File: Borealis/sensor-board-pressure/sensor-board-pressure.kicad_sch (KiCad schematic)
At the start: 3 parts, among them J1 Conn_01x06_Pin, J2 Conn_01x08_Pin (BMP390)

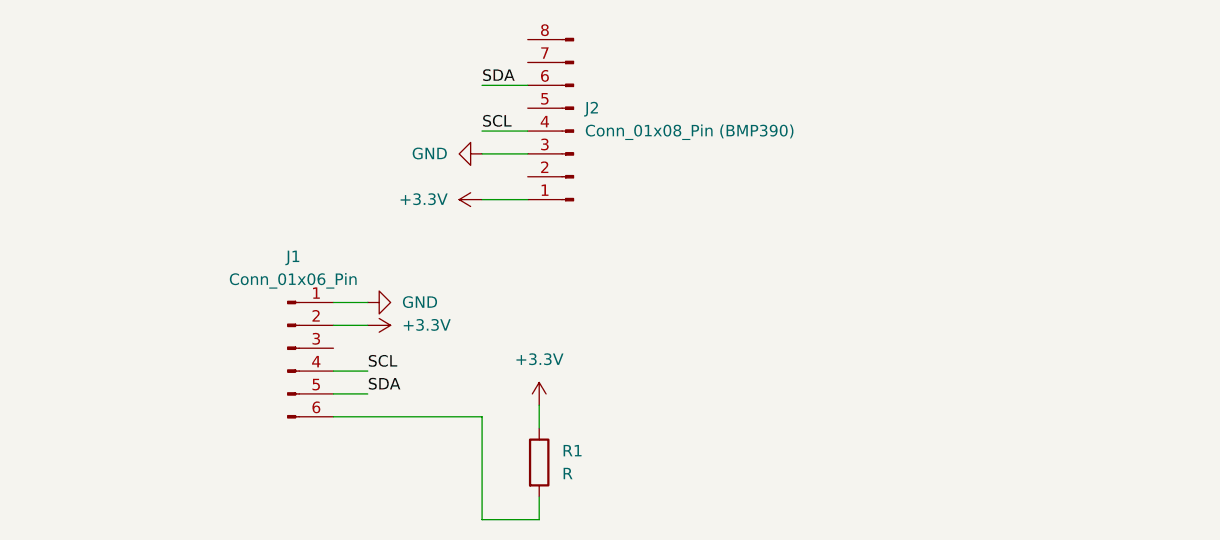
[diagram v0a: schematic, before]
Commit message: Updating changes
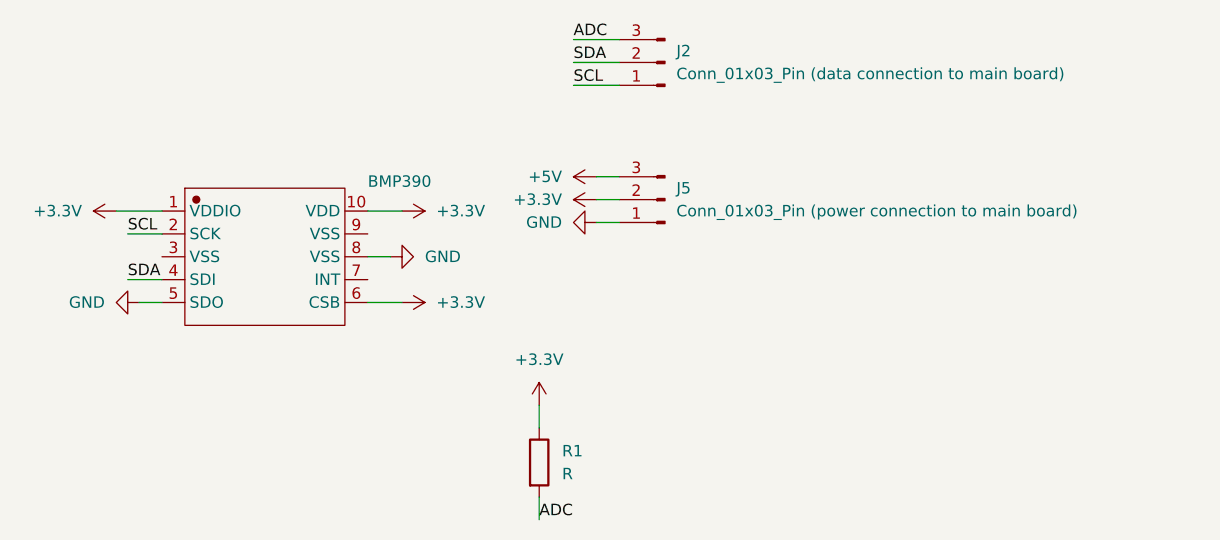
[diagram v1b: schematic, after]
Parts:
- removed J1: Conn_01x06_Pin, Connector_PinHeader_2.54mm:PinHeader_1x06_P2.54mm_Vertical, symbol Connector:Conn_01x06_Pin
- removed J2: Conn_01x08_Pin (BMP390), Adafruit BMP390:1X08_ROUND_70, symbol Connector:Conn_01x08_Pin
- added BMP390: ~, Adafruit BMP390:BMP388, symbol BMP390_2025-12-25-altium-import:root_0_BMP390_
- added J2: Conn_01x03_Pin (data connection to main board), batteryholder:1x03 2.3 pitch, symbol Connector:Conn_01x03_Pin
- added J5: Conn_01x03_Pin (power connection to main board), batteryholder:1x03 2.3 pitch, symbol Connector:Conn_01x03_Pin
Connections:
- net +3.3V: now also BMP390.1 (VDDIO), BMP390.10 (VDD), BMP390.6 (CSB), J5.2 (Pin_2)
- net GND: now also BMP390.5 (SDO), BMP390.8 (VSS), J5.1 (Pin_1)
- net SCL: now also BMP390.2 (SCK), J2.1 (Pin_1)
- net SDA: now also BMP390.4 (SDI), J2.2 (Pin_2)
- net ADC: now reaches R1.2
- net ADC: now also J2.3 (Pin_3)
- new net +5V: J5.3 (Pin_3)

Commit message: Added barometric sensor board
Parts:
- R1: footprint OptoDevice:R_LDR_4.9x4.2mm_P2.54mm_Vertical -> Resistor_SMD:R_0805_2012Metric
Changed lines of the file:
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@@
 			)
 		)
-		(property "Footprint" "OptoDevice:R_LDR_4.9x4.2mm_P2.54mm_Vertical"
+		(property "Footprint" "Resistor_SMD:R_0805_2012Metric"
 			(at 90.932 106.68 90)
 			(effects
